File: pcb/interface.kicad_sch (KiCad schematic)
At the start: 5 parts

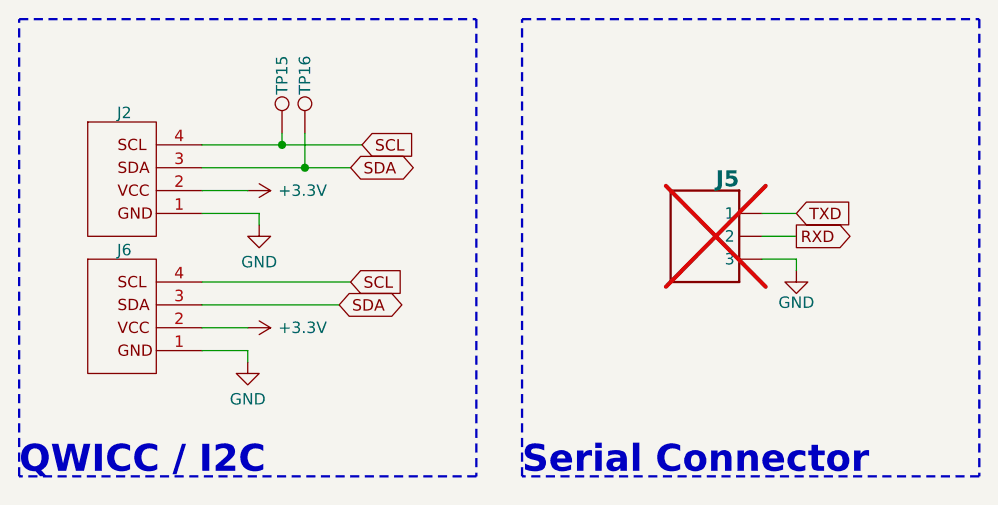
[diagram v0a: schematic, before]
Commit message: Updated for consistency with new patterns
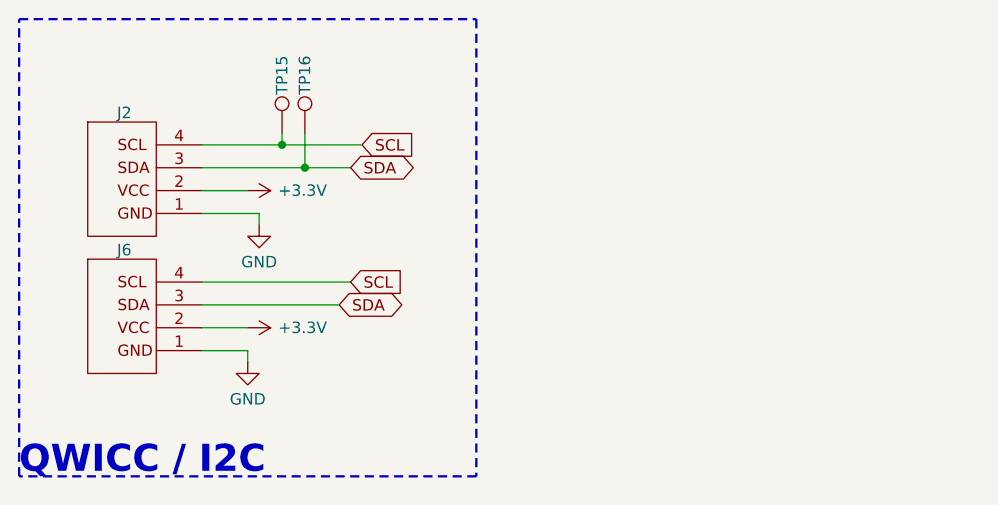
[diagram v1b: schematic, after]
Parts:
- removed J5: ~, CRGM Connector:JST_SH_BM03B-SRSS-TB_1x03-1MP_P1.00mm_Vertical, symbol CRGM Connector:JST-SH-3
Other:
- note removed: "Serial Connector"
